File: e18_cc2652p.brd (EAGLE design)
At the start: 14.8 x 23.4 mm, 45 parts, among them IC3 CC2652R1FRGZ, Q1 32.768kHz, U1 MX25R8035FZUIL0, Y1 Q22FA12800150

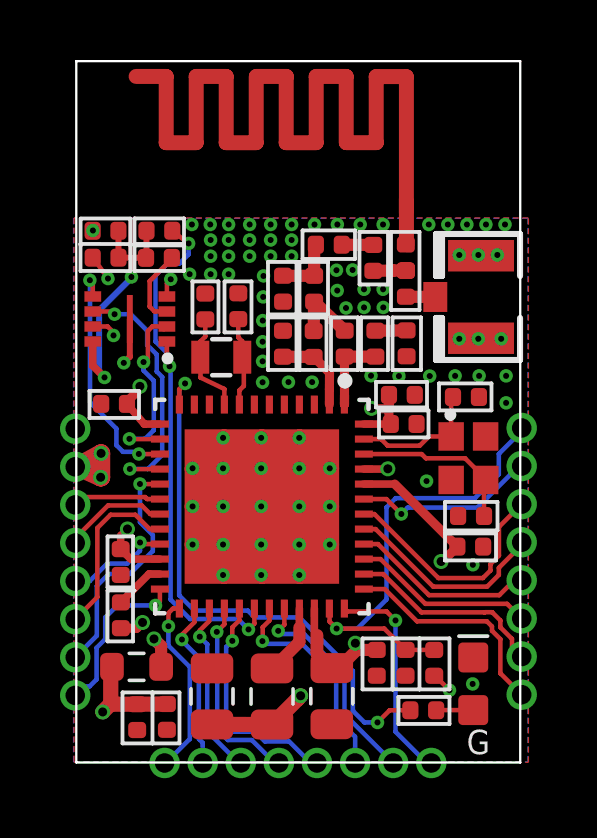
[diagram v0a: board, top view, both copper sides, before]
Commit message: Add files via upload
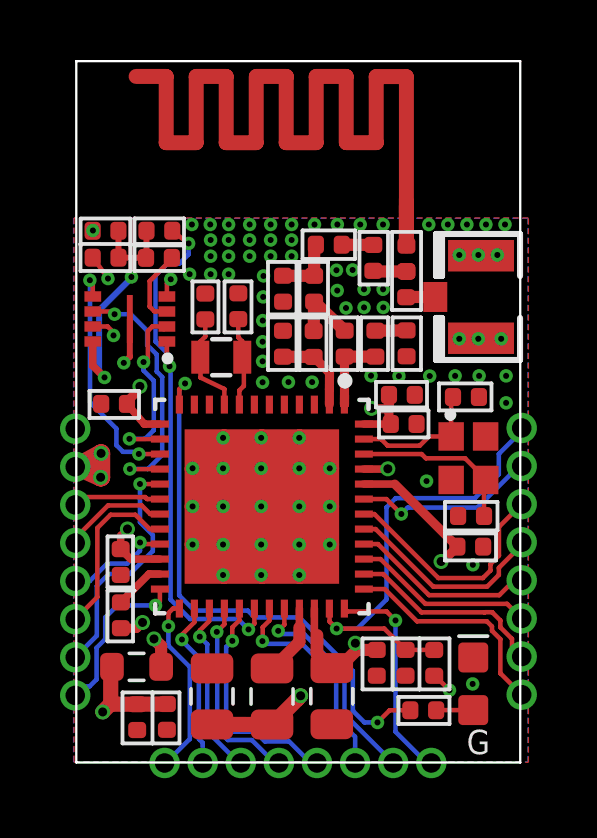
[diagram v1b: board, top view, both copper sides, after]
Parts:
- removed C21, C23: 1.8pf, discretes-dev:CAPC1005X40N
- added R6, R7: 0, ok-discretes-dev:_PKG_C_0402
- C19: value 12pf -> 2.2pf
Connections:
- net N$6: now also R7.2, X1.3; no longer C21.2, U$1.P$1, U$1.P$10, U$1.P$11, U$1.P$12, U$1.P$13, U$1.P$14, U$1.P$15, U$1.P$16, U$1.P$17, U$1.P$18, U$1.P$2, U$1.P$3, U$1.P$4, U$1.P$5, U$1.P$6, U$1.P$7, U$1.P$8, U$1.P$9, U$1.SIGNAL
- net N$7: now also R6.1, R7.1; no longer C21.1, C23.1
- net N$8: now also R6.2, U$1.P$1, U$1.P$10, U$1.P$11, U$1.P$12, U$1.P$13, U$1.P$14, U$1.P$15, U$1.P$16, U$1.P$17, U$1.P$18, U$1.P$2, U$1.P$3, U$1.P$4, U$1.P$5, U$1.P$6, U$1.P$7, U$1.P$8, U$1.P$9, U$1.SIGNAL; no longer C23.2, X1.3
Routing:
- net N$8: track 0.98 -> 36.9 mm
- net N$6: track 33.1 -> 0.97 mm
